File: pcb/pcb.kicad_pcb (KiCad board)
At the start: 2 copper layers, 21 parts, among them SW1 SW_Push, SW10 RotaryEncoder_Switch, SW2 SW_Push, SW3 SW_Push, SW4 SW_Push, SW5 SW_Push, SW6 SW_Push, SW7 SW_Push, SW8 SW_Push, SW9 SW_Push, U1 MOUDLE-SEEEDUINO-XIAO, U2 ER_OLEDM0.91_1x-I2C

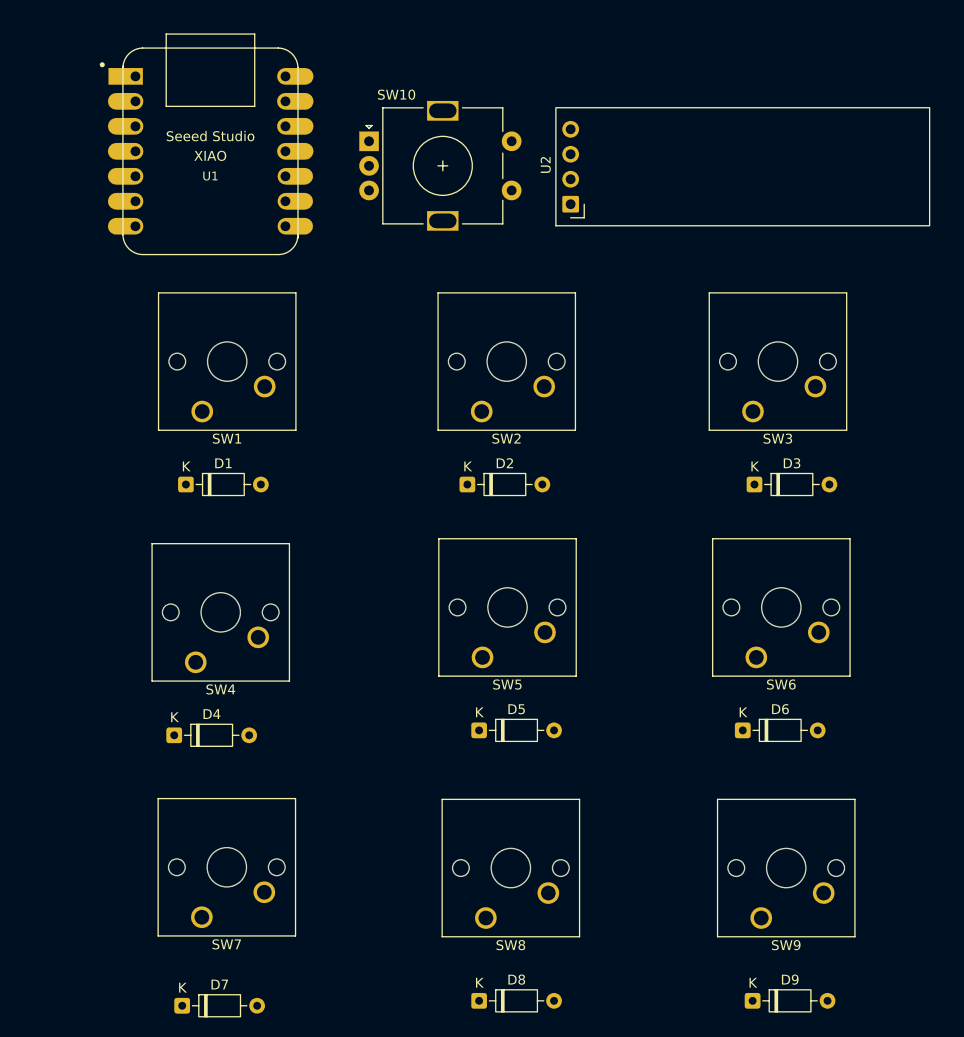
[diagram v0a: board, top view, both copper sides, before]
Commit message: routing on the pcb
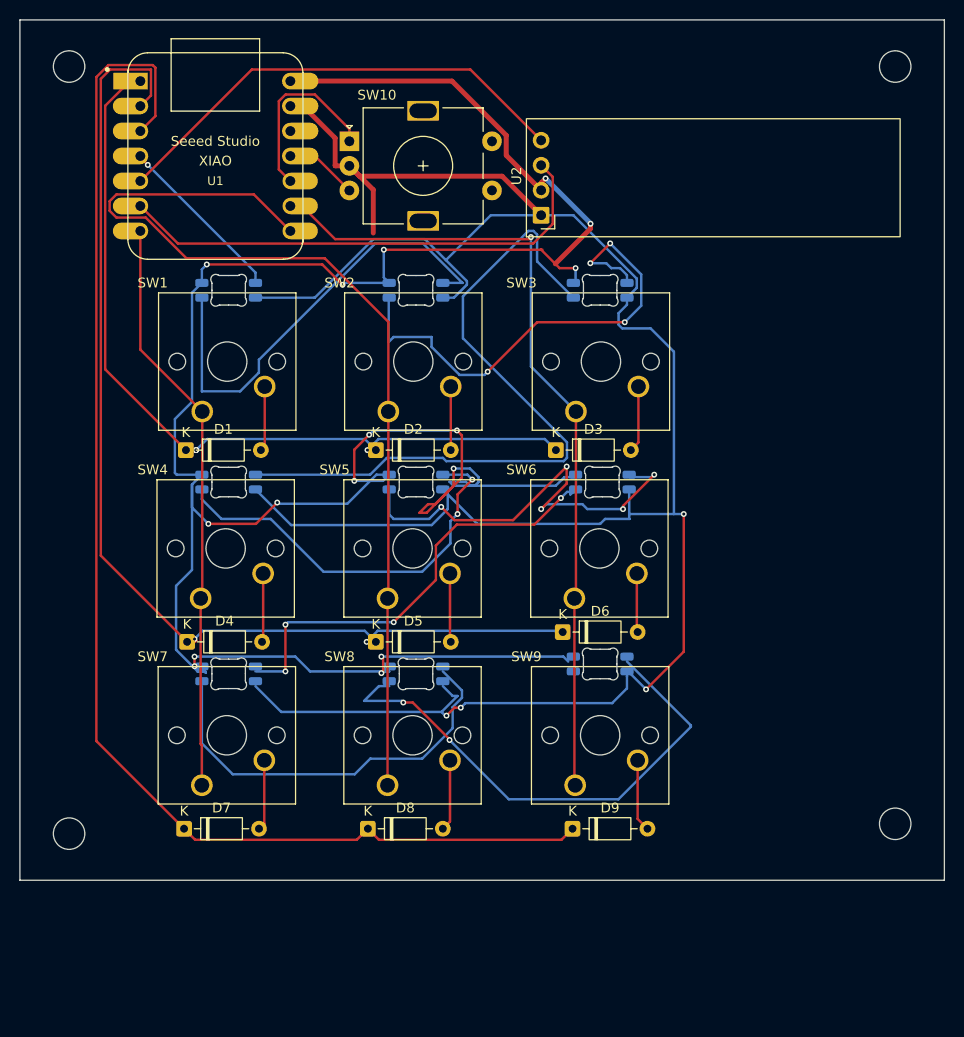
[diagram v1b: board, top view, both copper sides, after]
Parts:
- added D10: SK6812MINI-E, LED_SMD:LED_SK6812MINI-E_3.2x2.8mm_P1.5mm_ReverseMount, B.Cu at (92.2, 52.8)
- added D11: SK6812MINI-E, LED_SMD:LED_SK6812MINI-E_3.2x2.8mm_P1.5mm_ReverseMount, B.Cu at (111.3, 52.8)
- added D12: SK6812MINI-E, LED_SMD:LED_SK6812MINI-E_3.2x2.8mm_P1.5mm_ReverseMount, B.Cu at (130.0, 52.8)
- added D13: SK6812MINI-E, LED_SMD:LED_SK6812MINI-E_3.2x2.8mm_P1.5mm_ReverseMount, B.Cu at (92.2, 72.2)
- added D14: SK6812MINI-E, LED_SMD:LED_SK6812MINI-E_3.2x2.8mm_P1.5mm_ReverseMount, B.Cu at (111.3, 72.2)
- added D15: SK6812MINI-E, LED_SMD:LED_SK6812MINI-E_3.2x2.8mm_P1.5mm_ReverseMount, B.Cu at (130.2, 72.2)
- added D16: SK6812MINI-E, LED_SMD:LED_SK6812MINI-E_3.2x2.8mm_P1.5mm_ReverseMount, B.Cu at (92.2, 91.8)
- added D17: SK6812MINI-E, LED_SMD:LED_SK6812MINI-E_3.2x2.8mm_P1.5mm_ReverseMount, B.Cu at (111.3, 91.8)
- added D18: SK6812MINI-E, LED_SMD:LED_SK6812MINI-E_3.2x2.8mm_P1.5mm_ReverseMount, B.Cu at (130.0, 90.8)
- added H1: MountingHole, MountingHole:MountingHole_3.2mm_M3, F.Cu at (76.0, 30.0)
- added H2: MountingHole, MountingHole:MountingHole_3.2mm_M3, F.Cu at (76.0, 108.0)
- added H3: MountingHole, MountingHole:MountingHole_3.2mm_M3, F.Cu at (160.0, 30.0)
- added H3: MountingHole, MountingHole:MountingHole_3.2mm_M3, F.Cu at (160.0, 107.0)
- moved D9 25.3 mm to (127.2, 107.5)
- moved SW9 23.2 mm to (127.5, 103.1)
- moved D6 20.9 mm to (126.2, 87.5)
- moved D8 20.8 mm to (106.4, 107.5)
- moved D3 20.5 mm to (125.5, 69.0)
- moved SW6 19.4 mm to (127.4, 84.1)
- moved D7 18.0 mm to (87.7, 107.5)
- moved SW3 18.0 mm to (127.5, 65.1)
- moved SW8 16.8 mm to (108.4, 103.1)
- moved D5 13.8 mm to (107.2, 88.5)
- moved SW7 13.4 mm to (89.5, 103.1)
- moved SW5 11.4 mm to (108.4, 84.1)
- moved D2 9.95 mm to (107.2, 69.0)
- moved D4 9.59 mm to (88.0, 88.5)
- moved SW2 9.50 mm to (108.5, 65.1)
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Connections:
- SW10 pad S1: /RE3 -> unconnected-(SW10-PadS1)
- SW10 pad S2: GND -> unconnected-(SW10-PadS2)
- U1 pad 4: /RE3 -> /RGB
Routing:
- net VCC: track 0.00 -> 264.7 mm, vias 0 -> 16
- net GND: track 0.00 -> 242.6 mm, vias 0 -> 4
- net /R3: track 0.00 -> 135.2 mm
- net /R2: track 0.00 -> 112.4 mm, vias 0 -> 2
- net /C2: track 0.00 -> 101.3 mm
- net /R1: track 0.00 -> 84.2 mm, vias 0 -> 3
- net /C3: track 0.00 -> 83.9 mm, vias 0 -> 1
- net Net-(D12-DOUT): track 0.00 -> 71.9 mm
- net /C1: track 0.00 -> 59.1 mm
- net Net-(D17-DOUT): track 0.00 -> 53.0 mm, vias 0 -> 2
- net Net-(D11-DOUT): track 0.00 -> 51.0 mm, vias 0 -> 4
- net /SCL: track 0.00 -> 50.8 mm
- net /SDA: track 0.00 -> 48.4 mm
- net Net-(D10-DOUT): track 0.00 -> 46.7 mm
- net Net-(D15-DOUT): track 0.00 -> 46.2 mm, vias 0 -> 4
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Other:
- board outline added: 94 x 87.5 mm
